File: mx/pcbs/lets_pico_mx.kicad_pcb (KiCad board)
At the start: 2 copper layers, 114.1 x 80 mm, 30 parts, among them U0 Pico

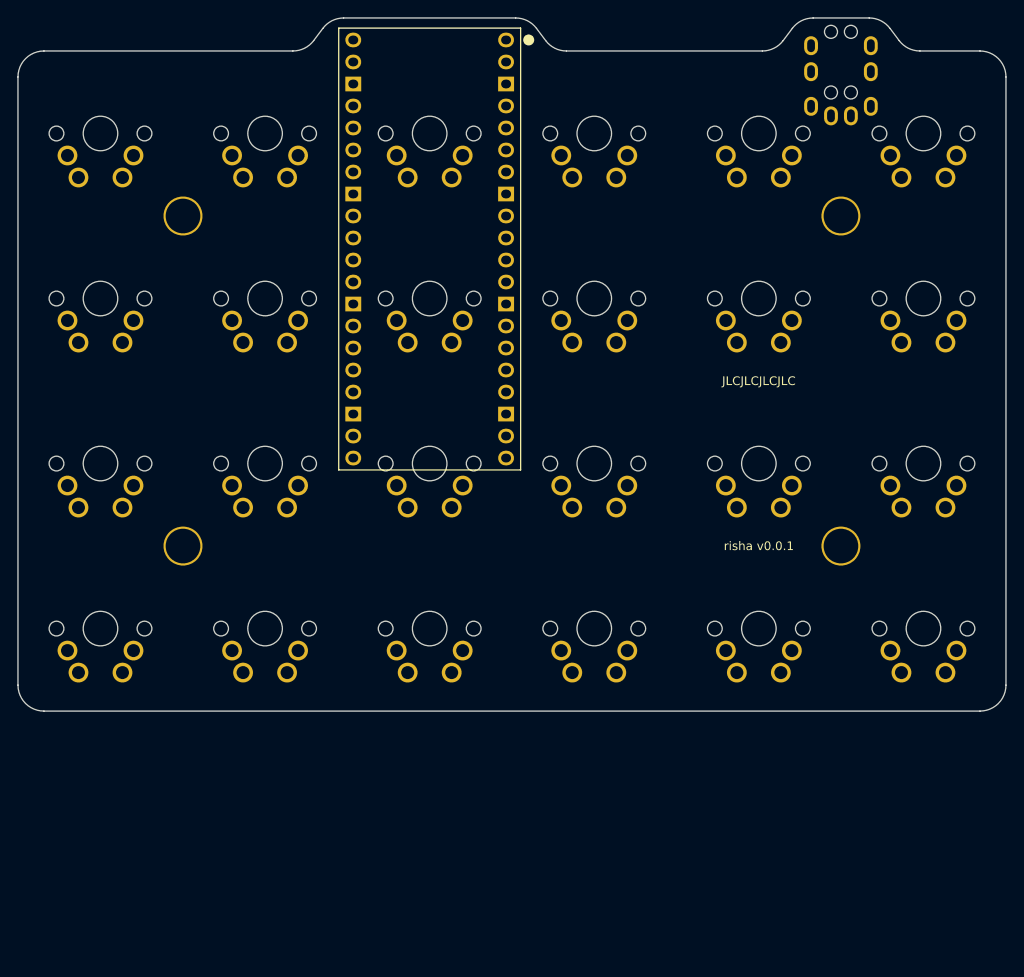
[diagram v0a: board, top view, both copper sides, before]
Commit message: rename
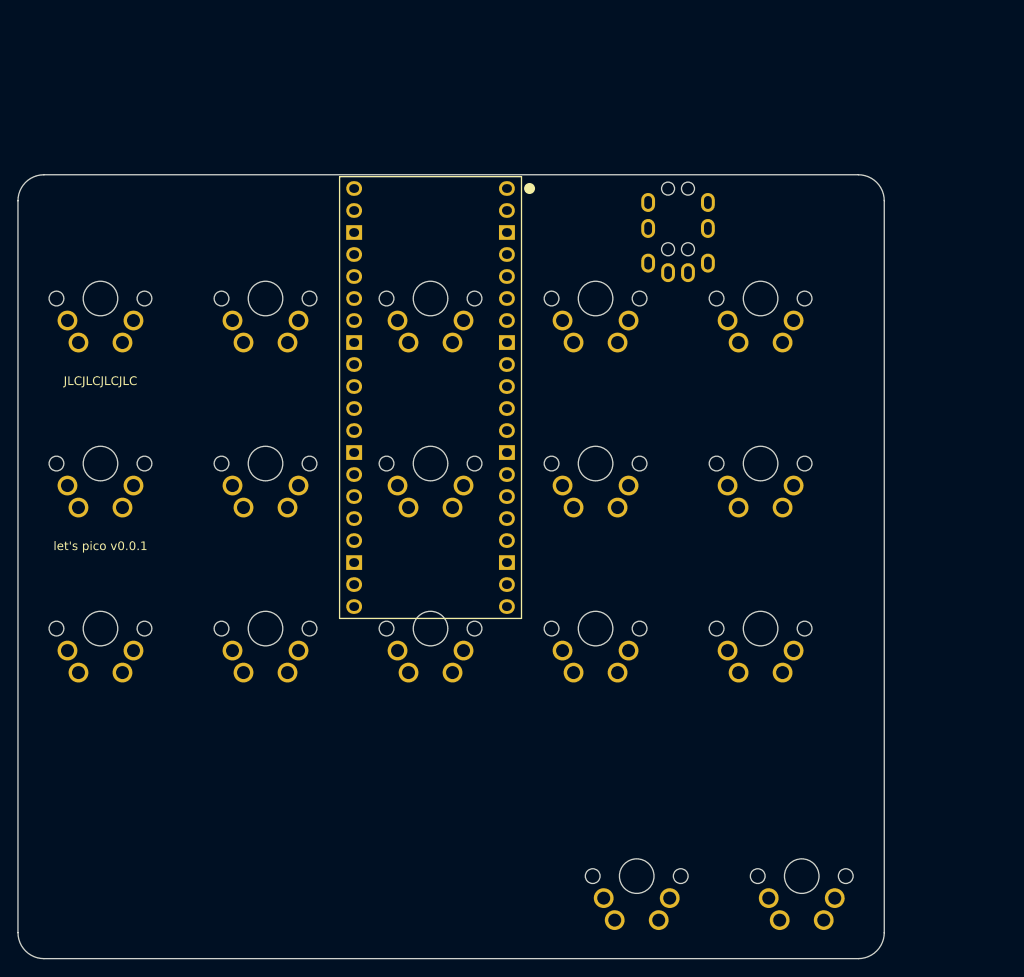
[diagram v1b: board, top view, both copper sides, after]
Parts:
- removed ? (x4): , DrillHole
- removed S18, S19, S20, S21, S22, S23, S24: , MX
- moved S16 85.9 mm to (214.3, 181.0)
- moved S4 60.2 mm to (171.5, 152.4)
- moved S7 42.6 mm to (190.5, 152.4)
- moved S8 42.6 mm to (190.5, 133.3)
- moved S9 38.1 mm to (190.5, 114.3)
- moved S17 29.0 mm to (233.4, 181.0)
- moved S10 27.0 mm to (209.6, 152.4)
- moved S11 27.0 mm to (209.6, 133.3)
- moved S12 27.0 mm to (209.6, 114.3)
- moved TRRS1 26.1 mm to (220.2, 100.0)
- moved S13 19.2 mm to (228.6, 152.4)
- moved S14 19.2 mm to (228.6, 133.3)
- moved S15 19.2 mm to (228.6, 114.3)
- moved S5 19.1 mm to (171.5, 133.3)
- moved S6 19.1 mm to (171.5, 114.3)
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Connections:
- net matrix_index_mod renamed thumbfan_far_home
- S1 pad 1: matrix_outer_mod -> matrix_pinky_bottom
- S10 pad 1: matrix_ring_bottom -> matrix_index_bottom
- S11 pad 1: matrix_ring_home -> matrix_index_home
- S12 pad 1: matrix_ring_top -> matrix_index_top
- S13 pad 1: matrix_middle_mod -> matrix_inner_bottom
- S14 pad 1: matrix_middle_bottom -> matrix_inner_home
- S15 pad 1: matrix_middle_home -> matrix_inner_top
- S16 pad 1: matrix_middle_top -> thumbfan_near_home
- S2 pad 1: matrix_outer_bottom -> matrix_pinky_home
- S3 pad 1: matrix_outer_home -> matrix_pinky_top
- S4 pad 1: matrix_outer_top -> matrix_ring_bottom
- S5 pad 1: matrix_pinky_mod -> matrix_ring_home
- S6 pad 1: matrix_pinky_bottom -> matrix_ring_top
- S7 pad 1: matrix_pinky_home -> matrix_middle_bottom
- S8 pad 1: matrix_pinky_top -> matrix_middle_home
- S9 pad 1: matrix_ring_mod -> matrix_middle_top
- TRRS1 pad 1: 3V3 -> VSYS
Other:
- board size 114.1 x 80 mm -> 100 x 90.5 mm
- board text added: "let's pico v0.0.1"
- board text removed: "risha v0.0.1"
